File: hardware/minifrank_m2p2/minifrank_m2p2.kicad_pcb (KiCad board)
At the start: 4 copper layers, 85.6 x 54 mm, 136 parts, among them J1 PWR, J10 VGA, J11 PJ-320D, J12 104031-0811, J2 UART, J3 DEBUG, J4 SS-52100-004, J5 USB4215-03-A, J6 MDC-036, J7 PJ-320D, J8 DC3RX19JA2, J9 GP2, U1 TS3USB221RSER, U10 ESP-01v090, U11 TDA1387T, U12 LM358, U2 USBLC6-2SC6, U3 MW7211A, U4 NCP1117-3.3_SOT223, U5 TXS0104ERGYR, U6 ESP-PSRAM32, U7 W25Q128JVS, U8 CD4069UBM, U9 RP2350, Y1 ASE-12MHz

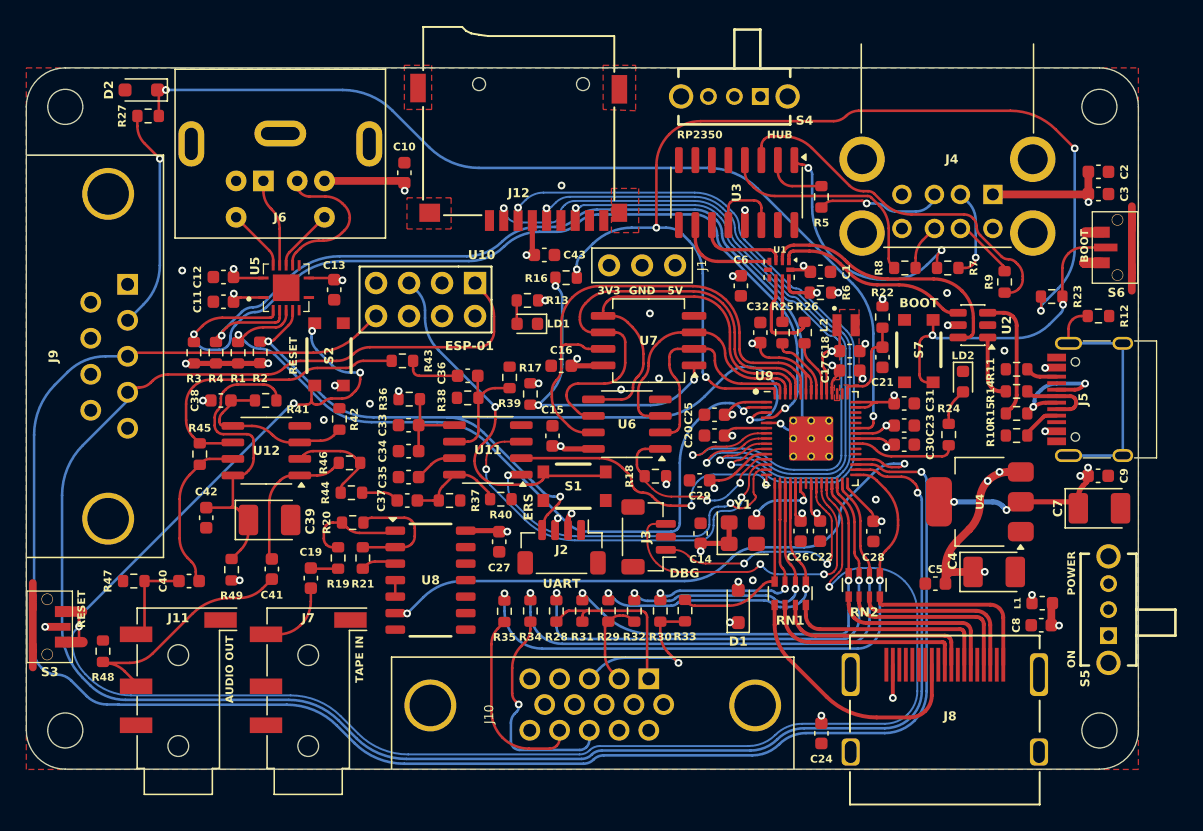
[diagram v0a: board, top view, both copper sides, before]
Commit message: Board updates
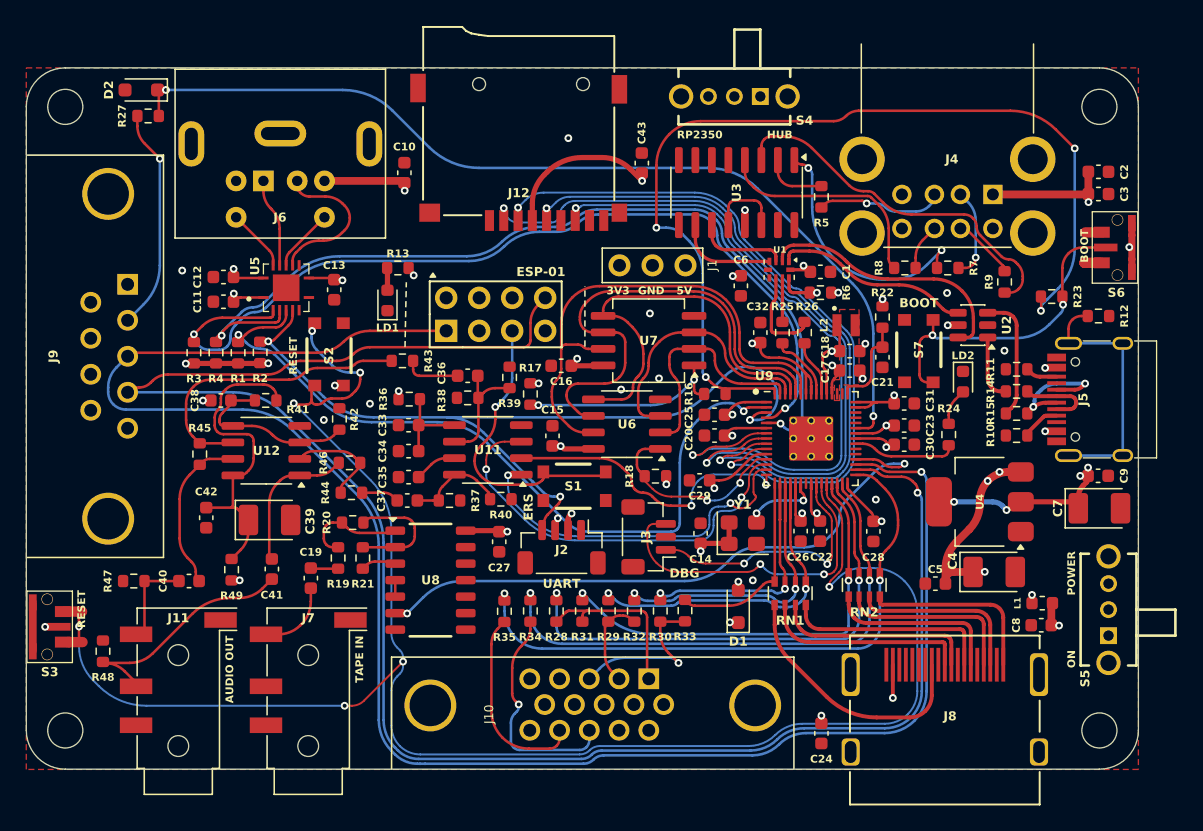
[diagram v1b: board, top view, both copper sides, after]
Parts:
- moved R16 14.5 mm to (183.7, 88.9)
- moved LD1 10.9 mm to (158.5, 81.7), turned to 90 degrees
- moved C43 10.3 mm to (178.1, 71.1), turned to -90 degrees
- moved R13 10.3 mm to (159.3, 79.2)
- moved U10 4.30 mm to (163.0, 84.0), turned to 90 degrees
- moved J1 0.80 mm to (176.4, 79.0)
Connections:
- U10 pad 1: /GPIO20 -> /GPIO21
- U10 pad 8: /GPIO21 -> /GPIO20
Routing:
- net +3V3: track 69.6 -> 79.9 mm
- net /RP2350A/FLASH_SS: track 23.7 -> 15.5 mm, vias 3 -> 2
- net /RP2350A/QSPI_SS: track 81.5 -> 73.9 mm, vias 5 -> 4
- net /GPIO21: track 143.4 -> 136.8 mm
- net /GPIO20: track 146.7 -> 140.6 mm
- net /RUN: track 139.9 -> 145.9 mm, vias 5 -> 7
- net GND: track 16.1 -> 10.1 mm, vias 16 -> 17
- net /ESP_RST: track 27.7 -> 22.0 mm
